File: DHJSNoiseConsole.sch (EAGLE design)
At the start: 11 parts

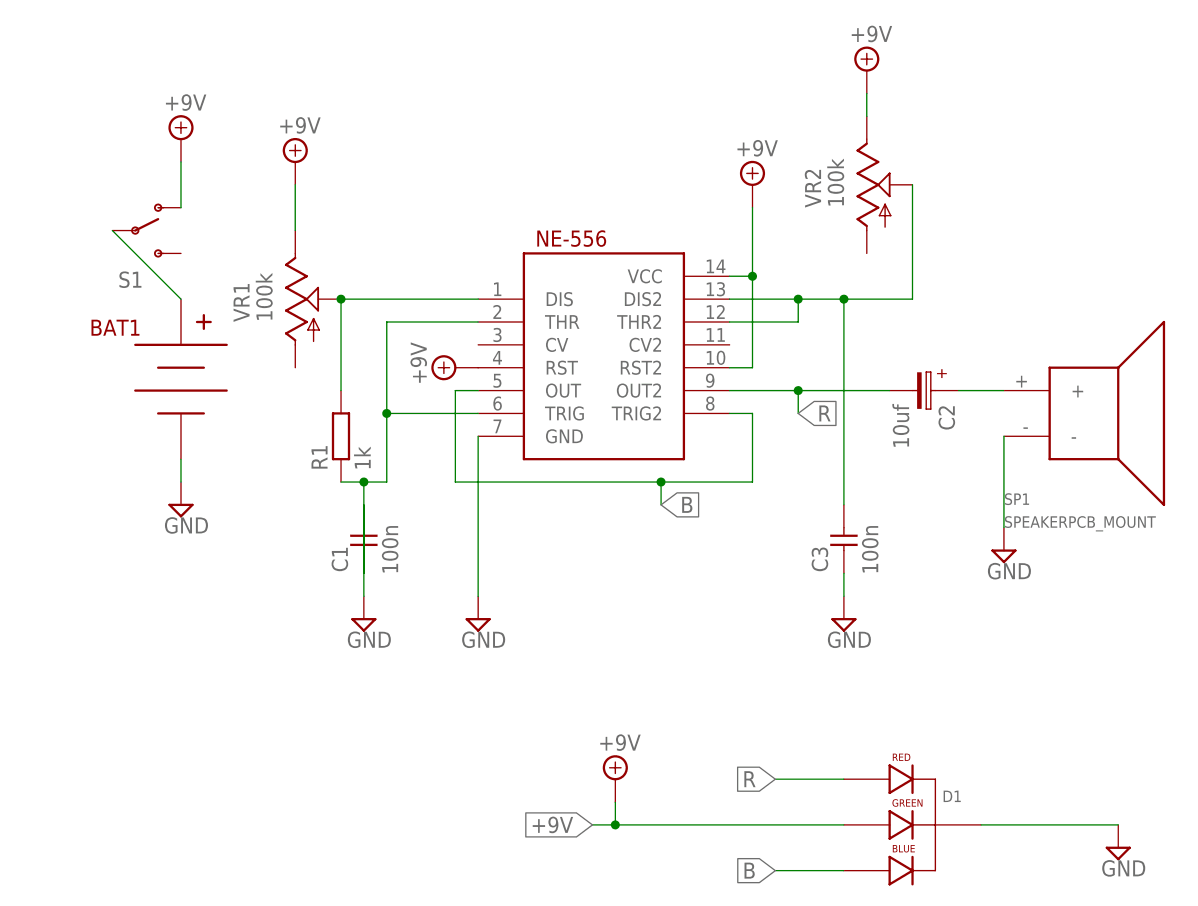
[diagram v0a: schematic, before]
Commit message: board
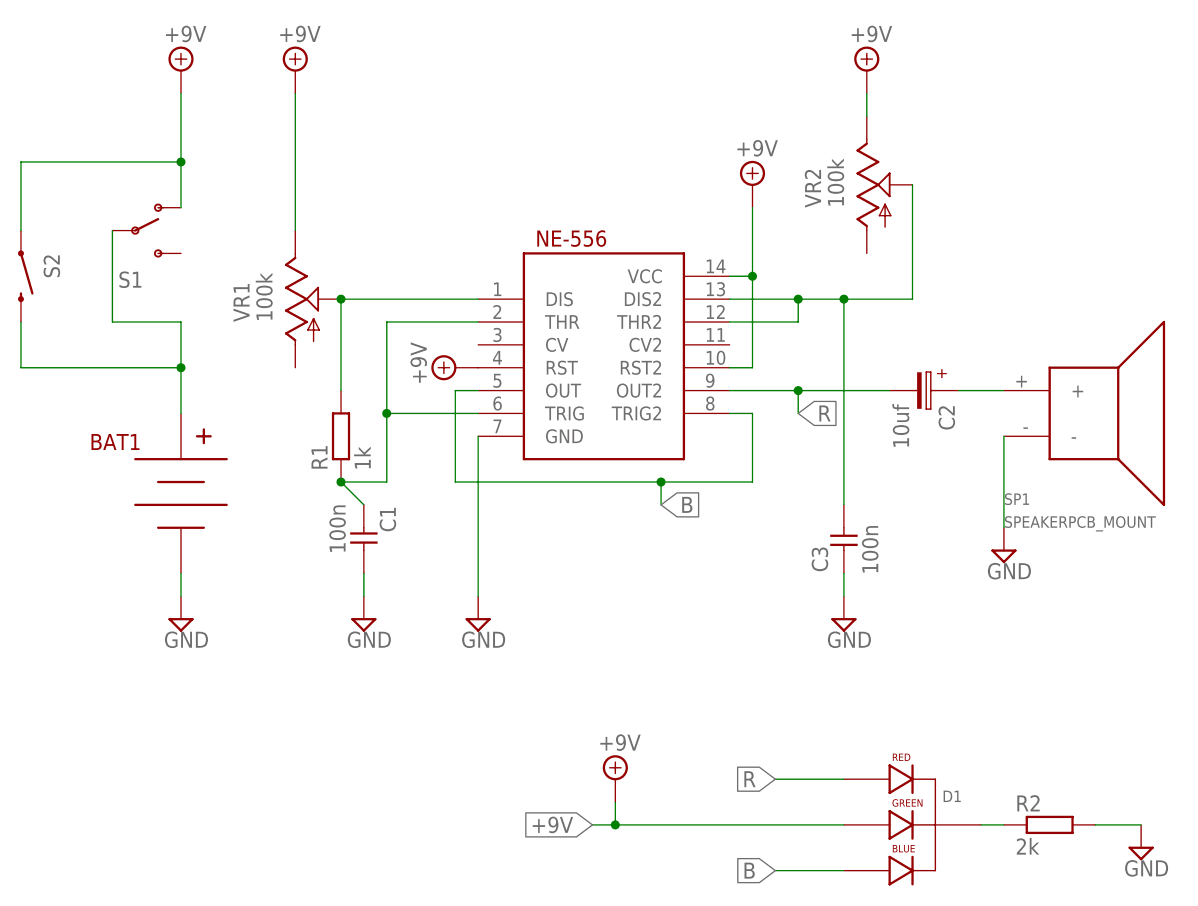
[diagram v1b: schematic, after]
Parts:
- added R2: 2k, MusicThingModular:RESISTOR10MM_RESISTOR
- added S2: SWITCH-MOMENTARY-2SIDE_EZ, SparkFun-Electromechanical:SWITCH-MOMENTARY-2SIDE_EZ
- VR1, VR2: device MusicThingModular:9MM_SNAP-IN_POTF2A -> MusicThingModular:9MM_SNAP-IN_POT_
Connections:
- new net N$4: D1.CATHODE, R2.1
- net +9V: now also S2.1
- net GND: now also R2.2; no longer D1.CATHODE
- net N$2: now also S2.2
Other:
- moved on the sheet: BAT1, C1
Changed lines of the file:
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@@
 <?xml version="1.0" encoding="utf-8"?>
 <!DOCTYPE eagle SYSTEM "eagle.dtd">
-<eagle version="7.2.0">
+<eagle version="6.6.0">
 <drawing>
 <settings>
@@
 </variantdefs>
 <classes>
-<class number="0" name="default" width="0" drill="0">
+<class number="0" name="default" width="0.6096" drill="0">
 </class>
 </classes>
 <parts>
-<part name="VR1" library="MusicThingModular" deviceset="9MM_SNAP-IN_POT" device="A" technology="F2" value="100k"/>
-<part name="VR2" library="MusicThingModular" deviceset="9MM_SNAP-IN_POT" device="A" technology="F2" value="100k"/>
+<part name="VR1" library="MusicThingModular" deviceset="9MM_SNAP-IN_POT" device="_" value="100k"/>
+<part name="VR2" library="MusicThingModular" deviceset="9MM_SNAP-IN_POT" device="_" value="100k"/>
 <part name="NE-556" library="SparkFun-AnalogIC" deviceset="556" device=""/>
 <part name="SUPPLY1" library="supply2" deviceset="+9V" device=""/>
@@
 <part name="SUPPLY11" library="supply2" deviceset="GND" device=""/>
 <part name="SUPPLY12" library="supply2" deviceset="+9V" device=""/>
+<part name="S2" library="SparkFun-Electromechanical" deviceset="SWITCH-MOMENTARY-2" device="SIDE_EZ" value=""/>
+<part name="R2" library="MusicThingModular" deviceset="RESISTOR" device="10MM_RESISTOR" value="2k"/>
 </parts>
 <sheets>
@@
 <instance part="VR2" gate="G$1" x="73.66" y="86.36"/>
 <instance part="NE-556" gate="G$1" x="43.18" y="68.58"/>
-<instance part="SUPPLY1" gate="G$1" x="10.16" y="88.9"/>
+<instance part="SUPPLY1" gate="G$1" x="10.16" y="99.06"/>
 <instance part="SP1" gate="G$1" x="99.06" y="60.96"/>
 <instance part="S1" gate="1" x="-7.62" y="81.28"/>
-<instance part="BAT1" gate="G$1" x="-2.54" y="66.04"/>
-<instance part="SUPPLY2" gate="G$1" x="-2.54" y="91.44"/>
-<instance part="SUPPLY3" gate="GND" x="-2.54" y="50.8"/>
+<instance part="BAT1" gate="G$1" x="-2.54" y="53.34"/>
+<instance part="SUPPLY2" gate="G$1" x="-2.54" y="99.06"/>
+<instance part="SUPPLY3" gate="GND" x="-2.54" y="38.1"/>
 <instance part="R1" gate="G$1" x="15.24" y="58.42" rot="R90"/>
 <instance part="SUPPLY4" gate="G$1" x="27.94" y="66.04" rot="R90"/>
-<instance part="C1" gate="G$1" x="17.78" y="48.26"/>
+<instance part="C1" gate="G$1" x="17.78" y="45.72" rot="R180"/>
 <instance part="C2" gate="G$1" x="78.74" y="63.5" rot="R270"/>
 <instance part="SUPPLY5" gate="GND" x="88.9" y="45.72"/>
@@
 <instance part="SUPPLY10" gate="GND" x="71.12" y="38.1"/>
 <instance part="D1" gate="G$1" x="76.2" y="15.24"/>
-<instance part="SUPPLY11" gate="GND" x="101.6" y="12.7"/>
+<instance part="SUPPLY11" gate="GND" x="104.14" y="12.7"/>
 <instance part="SUPPLY12" gate="G$1" x="45.72" y="20.32"/>
+<instance part="S2" gate="G$1" x="-20.32" y="76.2" rot="R270"/>
+<instance part="R2" gate="G$1" x="93.98" y="15.24"/>
 </instances>
 <busses>
@@
 <pinref part="VR1" gate="G$1" pin="E"/>
 <pinref part="SUPPLY1" gate="G$1" pin="+9V"/>
-<wire x1="10.16" y1="86.36" x2="10.16" y2="81.28" width="0.1524" layer="91"/>
+<wire x1="10.16" y1="96.52" x2="10.16" y2="81.28" width="0.1524" layer="91"/>
 </segment>
 <segment>
 <pinref part="S1" gate="1" pin="O"/>
 <pinref part="SUPPLY2" gate="G$1" pin="+9V"/>
+<wire x1="-2.54" y1="96.52" x2="-2.54" y2="88.9" width="0.1524" layer="91"/>
 <wire x1="-2.54" y1="88.9" x2="-2.54" y2="83.82" width="0.1524" layer="91"/>
+<wire x1="-20.32" y1="88.9" x2="-2.54" y2="88.9" width="0.1524" layer="91"/>
+<junction x="-2.54" y="88.9"/>
+<pinref part="S2" gate="G$1" pin="1"/>
+<wire x1="-20.32" y1="81.28" x2="-20.32" y2="88.9" width="0.1524" layer="91"/>
 </segment>
 <segment>
@@
 <pinref part="S1" gate="1" pin="P"/>
 <pinref part="BAT1" gate="G$1" pin="V+"/>
-<wire x1="-2.54" y1="73.66" x2="-10.16" y2="81.28" width="0.1524" layer="91"/>
+<wire x1="-2.54" y1="60.96" x2="-2.54" y2="66.04" width="0.1524" layer="91"/>
+<wire x1="-2.54" y1="66.04" x2="-2.54" y2="71.12" width="0.1524" layer="91"/>
+<wire x1="-2.54" y1="71.12" x2="-10.16" y2="71.12" width="0.1524" layer="91"/>
+<wire x1="-10.16" y1="71.12" x2="-10.16" y2="81.28" width="0.1524" layer="91"/>
+<wire x1="-20.32" y1="66.04" x2="-2.54" y2="66.04" width="0.1524" layer="91"/>
+<junction x="-2.54" y="66.04"/>
+<pinref part="S2" gate="G$1" pin="2"/>
+<wire x1="-20.32" y1="71.12" x2="-20.32" y2="66.04" width="0.1524" layer="91"/>
 </segment>
 </net>
@@
 <pinref part="BAT1" gate="G$1" pin="V-"/>
 <pinref part="SUPPLY3" gate="GND" pin="GND"/>
-<wire x1="-2.54" y1="53.34" x2="-2.54" y2="55.88" width="0.1524" layer="91"/>
+<wire x1="-2.54" y1="40.64" x2="-2.54" y2="43.18" width="0.1524" layer="91"/>
 </segment>
 <segment>
@@
 <pinref part="C1" gate="G$1" pin="1"/>
 <pinref part="SUPPLY7" gate="GND" pin="GND"/>
-<wire x1="17.78" y1="50.8" x2="17.78" y2="40.64" width="0.1524" layer="91"/>
+<wire x1="17.78" y1="43.18" x2="17.78" y2="40.64" width="0.1524" layer="91"/>
 </segment>
 <segment>
@@
 </segment>
 <segment>
-<pinref part="D1" gate="G$1" pin="CATHODE"/>
+<pinref part="R2" gate="G$1" pin="2"/>
 <pinref part="SUPPLY11" gate="GND" pin="GND"/>
-<wire x1="101.6" y1="15.24" x2="86.36" y2="15.24" width="0.1524" layer="91"/>
+<wire x1="104.14" y1="15.24" x2="99.06" y2="15.24" width="0.1524" layer="91"/>
 </segment>
 </net>
@@
 <segment>
 <pinref part="R1" gate="G$1" pin="1"/>
-<wire x1="20.32" y1="53.34" x2="17.78" y2="53.34" width="0.1524" layer="91"/>
+<wire x1="20.32" y1="53.34" x2="15.24" y2="53.34" width="0.1524" layer="91"/>
 <pinref part="NE-556" gate="G$1" pin="THR"/>
-<wire x1="17.78" y1="53.34" x2="15.24" y2="53.34" width="0.1524" layer="91"/>
 <wire x1="30.48" y1="71.12" x2="20.32" y2="71.12" width="0.1524" layer="91"/>
 <wire x1="20.32" y1="71.12" x2="20.32" y2="60.96" width="0.1524" layer="91"/>
@@
 <junction x="20.32" y="60.96"/>
 <pinref part="C1" gate="G$1" pin="2"/>
-<wire x1="17.78" y1="43.18" x2="17.78" y2="53.34" width="0.1524" layer="91"/>
-<junction x="17.78" y="53.34"/>
+<wire x1="17.78" y1="50.8" x2="15.24" y2="53.34" width="0.1524" layer="91"/>
+<junction x="15.24" y="53.34"/>
 </segment>
 </net>
@@
 </segment>
 </net>
+<net name="N$4" class="0">
+<segment>
+<pinref part="D1" gate="G$1" pin="CATHODE"/>
+<pinref part="R2" gate="G$1" pin="1"/>
+<wire x1="88.9" y1="15.24" x2="86.36" y2="15.24" width="0.1524" layer="91"/>
+</segment>
+</net>
